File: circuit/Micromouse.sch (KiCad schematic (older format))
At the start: 33 parts, among them J1 DBG_CN, J3 TEST_1P, J5 TEST_1P, J6 Conn_01x04, Q2 IRLML6344, SW2 SW_Push, SW3 SW_Push, SW4 SW_Push, U3 STM32F405RGTx

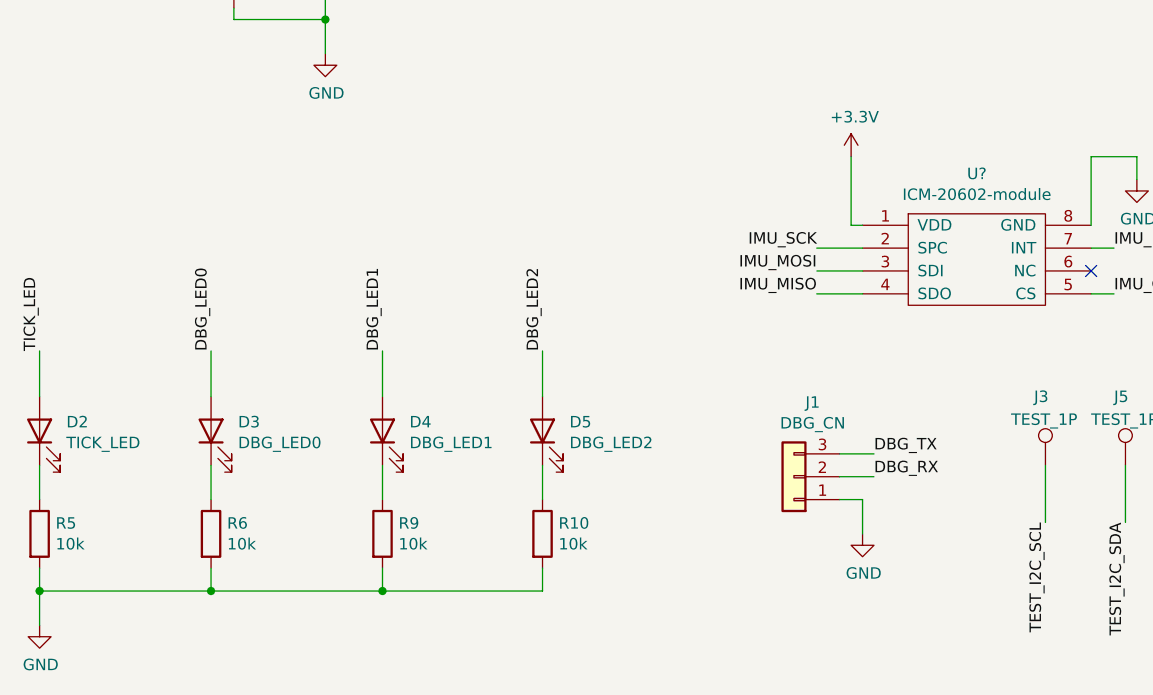
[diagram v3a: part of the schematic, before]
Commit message: ぽんぽんぺいん
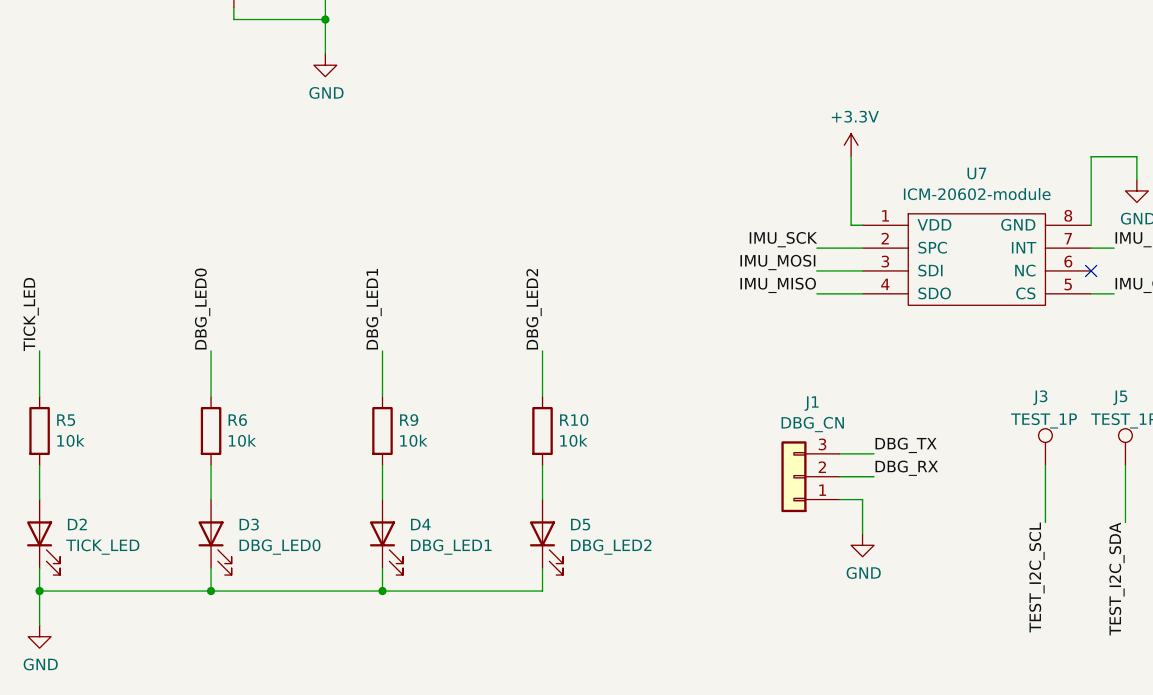
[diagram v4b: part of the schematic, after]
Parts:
- gave numbers to parts that had none: 1
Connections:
- net DBG_LED0: now also R6.1; no longer D3.2 (A)
- net DBG_LED1: now also R9.1; no longer D4.2 (A)
- net DBG_LED2: now also R10.1; no longer D5.2 (A)
- net GND: now also D2.1 (K), D3.1 (K), D4.1 (K), D5.1 (K); no longer R10.2, R5.2, R6.2, R9.2
- net TICK_LED: now also R5.1; no longer D2.2 (A)
- new net: D2.2 (A), R5.2
- new net: D3.2 (A), R6.2
- new net: D4.2 (A), R9.2
- new net: D5.2 (A), R10.2
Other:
- moved on the sheet: D2, D3, D4, D5, R10, R5, R6, R9
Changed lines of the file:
@@
 L Device:R R10
 U 1 1 5FA6B59C
+P 3600 9650
+F 0 "R10" H 3670 9696 50  0000 L CNN
+F 1 "10k" H 3670 9605 50  0000 L CNN
+F 2 "Resistor_SMD:R_0603_1608Metric" V 3530 9650 50  0001 C CNN
+F 3 "" H 3600 9650 50  0001 C CNN
+	1    3600 9650
+	1    0    0    -1
+$EndComp
+$Comp
+L Device:LED D5
+U 1 1 5FA6A60B
 P 3600 10100
-F 0 "R10" H 3670 10146 50  0000 L CNN
-F 1 "10k" H 3670 10055 50  0000 L CNN
-F 2 "Resistor_SMD:R_0603_1608Metric" V 3530 10100 50  0001 C CNN
+F 0 "D5" V 3639 9982 50  0000 R CNN
+F 1 "DBG_LED2" V 3548 9982 50  0000 R CNN
+F 2 "LED_SMD:LED_0603_1608Metric" H 3600 10100 50  0001 C CNN
 F 3 "" H 3600 10100 50  0001 C CNN
 	1    3600 10100
-	1    0    0    -1
-$EndComp
-$Comp
-L Device:LED D5
-U 1 1 5FA6A60B
-P 3600 9650
-F 0 "D5" V 3639 9532 50  0000 R CNN
-F 1 "DBG_LED2" V 3548 9532 50  0000 R CNN
-F 2 "LED_SMD:LED_0603_1608Metric" H 3600 9650 50  0001 C CNN
-F 3 "" H 3600 9650 50  0001 C CNN
-	1    3600 9650
 	0    -1   -1   0
 $EndComp
@@
 L Device:R R9
 U 1 1 5FA2C629
+P 2900 9650
+F 0 "R9" H 2970 9696 50  0000 L CNN
+F 1 "10k" H 2970 9605 50  0000 L CNN
+F 2 "Resistor_SMD:R_0603_1608Metric" V 2830 9650 50  0001 C CNN
+F 3 "" H 2900 9650 50  0001 C CNN
+	1    2900 9650
+	1    0    0    -1
+$EndComp
+$Comp
+L Device:R R6
+U 1 1 5FA2C1CC
+P 2150 9650
+F 0 "R6" H 2220 9696 50  0000 L CNN
+F 1 "10k" H 2220 9605 50  0000 L CNN
+F 2 "Resistor_SMD:R_0603_1608Metric" V 2080 9650 50  0001 C CNN
+F 3 "" H 2150 9650 50  0001 C CNN
+	1    2150 9650
+	1    0    0    -1
+$EndComp
+$Comp
+L Device:R R5
+U 1 1 5FA2BE4A
+P 1400 9650
+F 0 "R5" H 1470 9696 50  0000 L CNN
+F 1 "10k" H 1470 9605 50  0000 L CNN
+F 2 "Resistor_SMD:R_0603_1608Metric" V 1330 9650 50  0001 C CNN
+F 3 "" H 1400 9650 50  0001 C CNN
+	1    1400 9650
+	1    0    0    -1
+$EndComp
+$Comp
+L Device:LED D4
+U 1 1 5FA21915
 P 2900 10100
-F 0 "R9" H 2970 10146 50  0000 L CNN
-F 1 "10k" H 2970 10055 50  0000 L CNN
-F 2 "Resistor_SMD:R_0603_1608Metric" V 2830 10100 50  0001 C CNN
+F 0 "D4" V 2939 9982 50  0000 R CNN
+F 1 "DBG_LED1" V 2848 9982 50  0000 R CNN
+F 2 "LED_SMD:LED_0603_1608Metric" H 2900 10100 50  0001 C CNN
 F 3 "" H 2900 10100 50  0001 C CNN
 	1    2900 10100
-	1    0    0    -1
-$EndComp
-$Comp
-L Device:R R6
-U 1 1 5FA2C1CC
+	0    -1   -1   0
+$EndComp
+$Comp
+L Device:LED D3
+U 1 1 5FA21155
 P 2150 10100
-F 0 "R6" H 2220 10146 50  0000 L CNN
-F 1 "10k" H 2220 10055 50  0000 L CNN
-F 2 "Resistor_SMD:R_0603_1608Metric" V 2080 10100 50  0001 C CNN
+F 0 "D3" V 2189 9982 50  0000 R CNN
+F 1 "DBG_LED0" V 2098 9982 50  0000 R CNN
+F 2 "LED_SMD:LED_0603_1608Metric" H 2150 10100 50  0001 C CNN
 F 3 "" H 2150 10100 50  0001 C CNN
 	1    2150 10100
-	1    0    0    -1
-$EndComp
-$Comp
-L Device:R R5
-U 1 1 5FA2BE4A
+	0    -1   -1   0
+$EndComp
+$Comp
+L Device:LED D2
+U 1 1 5FA206BB
 P 1400 10100
-F 0 "R5" H 1470 10146 50  0000 L CNN
-F 1 "10k" H 1470 10055 50  0000 L CNN
-F 2 "Resistor_SMD:R_0603_1608Metric" V 1330 10100 50  0001 C CNN
+F 0 "D2" V 1439 9983 50  0000 R CNN
+F 1 "TICK_LED" V 1348 9983 50  0000 R CNN
+F 2 "LED_SMD:LED_0603_1608Metric" H 1400 10100 50  0001 C CNN
 F 3 "" H 1400 10100 50  0001 C CNN
 	1    1400 10100
-	1    0    0    -1
-$EndComp
-$Comp
-L Device:LED D4
-U 1 1 5FA21915
-P 2900 9650
-F 0 "D4" V 2939 9532 50  0000 R CNN
-F 1 "DBG_LED1" V 2848 9532 50  0000 R CNN
-F 2 "LED_SMD:LED_0603_1608Metric" H 2900 9650 50  0001 C CNN
-F 3 "" H 2900 9650 50  0001 C CNN
-	1    2900 9650
-	0    -1   -1   0
-$EndComp
-$Comp
-L Device:LED D3
-U 1 1 5FA21155
-P 2150 9650
-F 0 "D3" V 2189 9532 50  0000 R CNN
-F 1 "DBG_LED0" V 2098 9532 50  0000 R CNN
-F 2 "LED_SMD:LED_0603_1608Metric" H 2150 9650 50  0001 C CNN
-F 3 "" H 2150 9650 50  0001 C CNN
-	1    2150 9650
-	0    -1   -1   0
-$EndComp
-$Comp
-L Device:LED D2
-U 1 1 5FA206BB
-P 1400 9650
-F 0 "D2" V 1439 9533 50  0000 R CNN
-F 1 "TICK_LED" V 1348 9533 50  0000 R CNN
-F 2 "LED_SMD:LED_0603_1608Metric" H 1400 9650 50  0001 C CNN
-F 3 "" H 1400 9650 50  0001 C CNN
-	1    1400 9650
 	0    -1   -1   0
 $EndComp
@@
 $EndComp
 $Comp
-L Sensor_Motion:ICM-20602-module U?
+L Sensor_Motion:ICM-20602-module U7
 U 1 1 5FBFC8AB
 P 5500 8900
-F 0 "U?" H 5500 9275 50  0000 C CNN
+F 0 "U7" H 5500 9275 50  0000 C CNN
 F 1 "ICM-20602-module" H 5500 9184 50  0000 C CNN
 F 2 "Original:ICM-20602" H 5500 8900 50  0001 C CNN
